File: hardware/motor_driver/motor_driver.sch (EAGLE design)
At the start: 84 parts

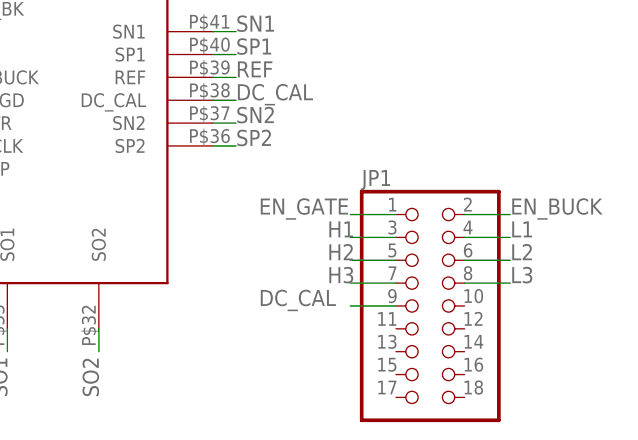
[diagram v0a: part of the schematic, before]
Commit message: Pushing library updates
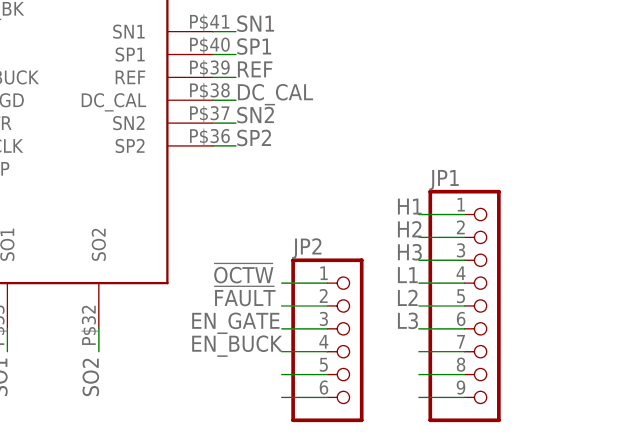
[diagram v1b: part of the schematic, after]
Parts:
- added JP2: (no value), adafruit:PINHD-1X6
- JP1: device adafruit:PINHD-2X9-CBIG -> adafruit:PINHD-1X9
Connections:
- new net N$13: JP2.5
- new net N$14: JP2.6
- new net N$17: JP1.7
- new net N$18: JP1.8
- new net N$19: JP1.9
- net !FAULT: now also JP2.2
- net !OCTW: now also JP2.1
- net DC_CAL: no longer JP1.9
- net EN_BUCK: now also JP2.4; no longer JP1.2
- net EN_GATE: now also JP2.3; no longer JP1.1
- net H1: now also JP1.1; no longer JP1.3
- net H2: now also JP1.2; no longer JP1.5
- net H3: now also JP1.3; no longer JP1.7
- net L2: now also JP1.5; no longer JP1.6
- net L3: now also JP1.6; no longer JP1.8
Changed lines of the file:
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@@
 <part name="C28" library="adafruit" deviceset="C-US" device="C1206" value="1n"/>
 <part name="R36" library="adafruit" deviceset="R-US_" device="R0805" value="10m"/>
-<part name="JP1" library="adafruit" deviceset="PINHD-2X9" device="-CBIG"/>
+<part name="JP1" library="adafruit" deviceset="PINHD-1X9" device=""/>
+<part name="JP2" library="adafruit" deviceset="PINHD-1X6" device=""/>
 </parts>
 <sheets>
@@
 <instance part="C28" gate="G$1" x="129.54" y="66.04"/>
 <instance part="R36" gate="G$1" x="139.7" y="66.04" rot="R270"/>
-<instance part="JP1" gate="A" x="231.14" y="22.86"/>
+<instance part="JP1" gate="G$1" x="238.76" y="22.86"/>
+<instance part="JP2" gate="A" x="223.52" y="17.78"/>
 </instances>
 <busses>
@@
 </segment>
 <segment>
-<pinref part="JP1" gate="A" pin="1"/>
-<wire x1="228.6" y1="33.02" x2="223.52" y2="33.02" width="0.1524" layer="91"/>
-<label x="213.36" y="33.02" size="1.778" layer="95"/>
+<pinref part="JP2" gate="A" pin="3"/>
+<wire x1="220.98" y1="20.32" x2="215.9" y2="20.32" width="0.1524" layer="91"/>
+<label x="205.74" y="20.32" size="1.778" layer="95"/>
 </segment>
 </net>
@@
 </segment>
 <segment>
-<pinref part="JP1" gate="A" pin="3"/>
-<wire x1="228.6" y1="30.48" x2="223.52" y2="30.48" width="0.1524" layer="91"/>
-<label x="220.98" y="30.48" size="1.778" layer="95"/>
+<pinref part="JP1" gate="G$1" pin="1"/>
+<wire x1="236.22" y1="33.02" x2="231.14" y2="33.02" width="0.1524" layer="91"/>
+<label x="228.6" y="33.02" size="1.778" layer="95"/>
 </segment>
 </net>
@@
 </segment>
 <segment>
-<pinref part="JP1" gate="A" pin="4"/>
-<wire x1="236.22" y1="30.48" x2="241.3" y2="30.48" width="0.1524" layer="91"/>
-<label x="241.3" y="30.48" size="1.778" layer="95"/>
+<pinref part="JP1" gate="G$1" pin="4"/>
+<wire x1="236.22" y1="25.4" x2="231.14" y2="25.4" width="0.1524" layer="91"/>
+<label x="228.6" y="25.4" size="1.778" layer="95"/>
 </segment>
 </net>
@@
 </segment>
 <segment>
-<pinref part="JP1" gate="A" pin="5"/>
-<wire x1="228.6" y1="27.94" x2="223.52" y2="27.94" width="0.1524" layer="91"/>
-<label x="220.98" y="27.94" size="1.778" layer="95"/>
+<pinref part="JP1" gate="G$1" pin="2"/>
+<wire x1="236.22" y1="30.48" x2="231.14" y2="30.48" width="0.1524" layer="91"/>
+<label x="228.6" y="30.48" size="1.778" layer="95"/>
 </segment>
 </net>
@@
 </segment>
 <segment>
-<pinref part="JP1" gate="A" pin="6"/>
-<wire x1="236.22" y1="27.94" x2="241.3" y2="27.94" width="0.1524" layer="91"/>
-<label x="241.3" y="27.94" size="1.778" layer="95"/>
+<pinref part="JP1" gate="G$1" pin="5"/>
+<wire x1="236.22" y1="22.86" x2="231.14" y2="22.86" width="0.1524" layer="91"/>
+<label x="228.6" y="22.86" size="1.778" layer="95"/>
 </segment>
 </net>
@@
 </segment>
 <segment>
-<pinref part="JP1" gate="A" pin="7"/>
-<wire x1="228.6" y1="25.4" x2="223.52" y2="25.4" width="0.1524" layer="91"/>
-<label x="220.98" y="25.4" size="1.778" layer="95"/>
+<pinref part="JP1" gate="G$1" pin="3"/>
+<wire x1="236.22" y1="27.94" x2="231.14" y2="27.94" width="0.1524" layer="91"/>
+<label x="228.6" y="27.94" size="1.778" layer="95"/>
 </segment>
 </net>
@@
 </segment>
 <segment>
-<pinref part="JP1" gate="A" pin="8"/>
-<wire x1="236.22" y1="25.4" x2="241.3" y2="25.4" width="0.1524" layer="91"/>
-<label x="241.3" y="25.4" size="1.778" layer="95"/>
+<pinref part="JP1" gate="G$1" pin="6"/>
+<wire x1="231.14" y1="20.32" x2="236.22" y2="20.32" width="0.1524" layer="91"/>
+<label x="228.6" y="20.32" size="1.778" layer="95"/>
 </segment>
 </net>
@@
 </segment>
 <segment>
-<pinref part="JP1" gate="A" pin="2"/>
-<wire x1="236.22" y1="33.02" x2="241.3" y2="33.02" width="0.1524" layer="91"/>
-<label x="241.3" y="33.02" size="1.778" layer="95"/>
+<pinref part="JP2" gate="A" pin="4"/>
+<wire x1="220.98" y1="17.78" x2="215.9" y2="17.78" width="0.1524" layer="91"/>
+<label x="205.74" y="17.78" size="1.778" layer="95"/>
 </segment>
 </net>
@@
 <wire x1="208.28" y1="45.72" x2="210.82" y2="45.72" width="0.1524" layer="91"/>
 <label x="210.82" y="45.72" size="1.778" layer="95"/>
-</segment>
-<segment>
-<pinref part="JP1" gate="A" pin="9"/>
-<wire x1="228.6" y1="22.86" x2="223.52" y2="22.86" width="0.1524" layer="91"/>
-<label x="213.36" y="22.86" size="1.778" layer="95"/>
 </segment>
 </net>
@@
 <label x="170.18" y="114.3" size="1.778" layer="95" rot="R180"/>
 </segment>
+<segment>
+<pinref part="JP2" gate="A" pin="1"/>
+<wire x1="220.98" y1="25.4" x2="215.9" y2="25.4" width="0.1524" layer="91"/>
+<label x="208.28" y="25.4" size="1.778" layer="95"/>
+</segment>
 </net>
 <net name="!FAULT" class="0">
@@
 <wire x1="172.72" y1="109.22" x2="170.18" y2="109.22" width="0.1524" layer="91"/>
 <label x="170.18" y="111.76" size="1.778" layer="95" rot="R180"/>
+</segment>
+<segment>
+<pinref part="JP2" gate="A" pin="2"/>
+<wire x1="220.98" y1="22.86" x2="215.9" y2="22.86" width="0.1524" layer="91"/>
+<label x="208.28" y="22.86" size="1.778" layer="95"/>
 </segment>
 </net>
@@
 </segment>
 </net>
+<net name="N$17" class="0">
+<segment>
+<pinref part="JP1" gate="G$1" pin="7"/>
+<wire x1="236.22" y1="17.78" x2="231.14" y2="17.78" width="0.1524" layer="91"/>
+</segment>
+</net>
+<net name="N$18" class="0">
+<segment>
+<pinref part="JP1" gate="G$1" pin="8"/>
+<wire x1="236.22" y1="15.24" x2="231.14" y2="15.24" width="0.1524" layer="91"/>
+</segment>
+</net>
+<net name="N$19" class="0">
+<segment>
+<pinref part="JP1" gate="G$1" pin="9"/>
+<wire x1="236.22" y1="12.7" x2="231.14" y2="12.7" width="0.1524" layer="91"/>
+</segment>
+</net>
+<net name="N$13" class="0">
+<segment>
+<pinref part="JP2" gate="A" pin="5"/>
+<wire x1="220.98" y1="15.24" x2="215.9" y2="15.24" width="0.1524" layer="91"/>
+</segment>
+</net>
+<net name="N$14" class="0">
+<segment>
+<pinref part="JP2" gate="A" pin="6"/>
+<wire x1="220.98" y1="12.7" x2="215.9" y2="12.7" width="0.1524" layer="91"/>
+</segment>
+</net>
